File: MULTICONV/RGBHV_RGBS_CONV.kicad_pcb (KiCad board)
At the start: 2 copper layers, 100 x 100 mm, 111 parts, among them J1 DIGITAL RGB, J10 AUDIO1, J11 RGBHV_2, J12 AUDIO2, J15 RGBS_OUT1, J16 RGBS_OUT2, J17 VIN, J2 VGA DB15, J3 ANALOG RGB DA15, J4 X1, J5 DIGITAL_RGBHV_1, J6 ANALOG RGB, J7 DIGITAL_RGBHV_2, J8 SWITCHER, J9 RGBHV_1, U1 OUT_GND_IN_3.3V, U2 74HC86, U3 OUT_IN_GND_3.3V, U4 IN_OUT_GND_3.3V

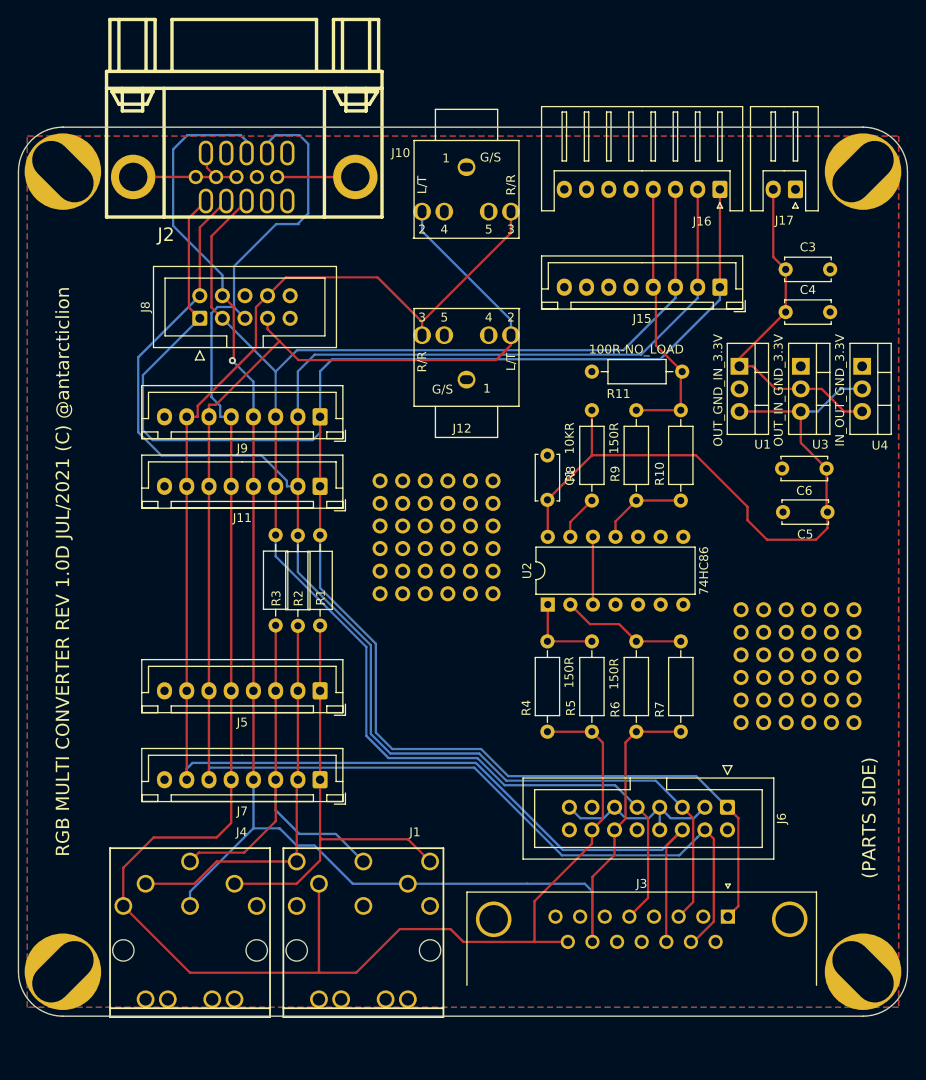
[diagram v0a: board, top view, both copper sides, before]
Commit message: Rev1.5 リリース候補
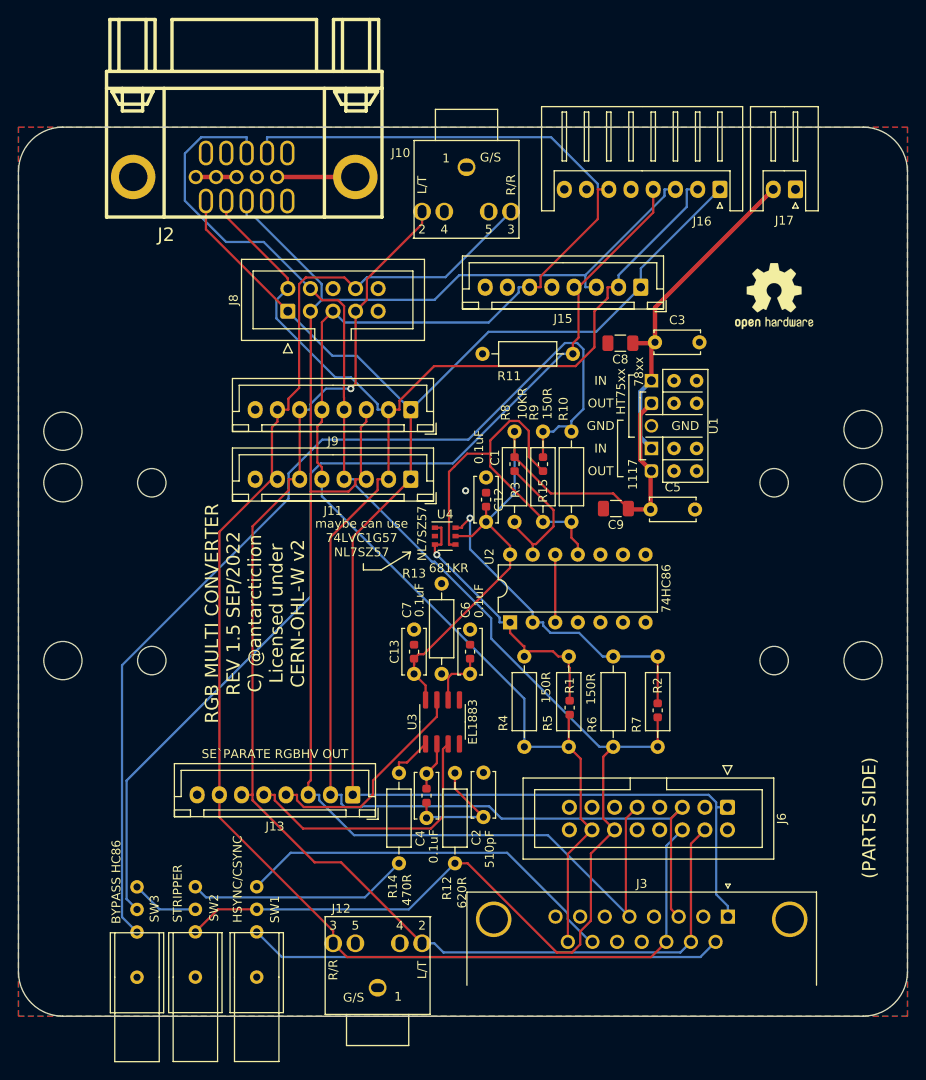
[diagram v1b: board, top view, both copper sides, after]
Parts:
- removed J1: DIGITAL RGB, ryuk_lib:DIN 8 PCB
- removed J4: X1, ryuk_lib:DIN_6_PCB
- removed J5: DIGITAL_RGBHV_1, Connector_JST:JST_XH_B8B-XH-A_1x08_P2.50mm_Vertical
- removed J7: DIGITAL_RGBHV_2, Connector_JST:JST_XH_B8B-XH-A_1x08_P2.50mm_Vertical
- removed PIN01 (x2), PIN02 (x2), PIN03 (x2), PIN04 (x2), PIN05 (x2), PIN06 (x2), PIN07 (x2), PIN08 (x2), PIN09 (x2), PIN10 (x2), PIN11 (x2), PIN12 (x2), PIN13 (x2), PIN14 (x2), PIN15 (x2), PIN16 (x2), PIN17 (x2), PIN18 (x2), PIN19 (x2), PIN20 (x2), PIN21 (x2), PIN22 (x2), PIN23 (x2), PIN24 (x2), PIN25 (x2), PIN26 (x2), PIN27 (x2), PIN28 (x2), PIN29 (x2), PIN30 (x2), PIN31 (x2), PIN32 (x2), PIN33 (x2), PIN34 (x2), PIN35 (x2), PIN36 (x2): Pin_2.54, ryuk_lib:Pin_2.54
- added C10: 0.1uF, Capacitor_SMD:C_0603_1608Metric, F.Cu at (95.9, 137.2)
- added C11: 0.1uF, Capacitor_SMD:C_0603_1608Metric, F.Cu at (100.8, 121.0)
- added C12: 0.1uF, Capacitor_SMD:C_0603_1608Metric, F.Cu at (102.6, 103.9)
- added C13: 0.1uF, Capacitor_SMD:C_0603_1608Metric, F.Cu at (94.5, 121.0)
- added C2: 510pF, Capacitor_THT:C_Disc_D5.0mm_W2.5mm_P5.00mm, F.Cu at (102.3, 139.6)
- added C7: 0.1uF, Capacitor_THT:C_Disc_D5.0mm_W2.5mm_P5.00mm, F.Cu at (94.5, 118.5)
- added C8: 10uF, Capacitor_SMD:C_1206_3216Metric, F.Cu at (117.7, 86.3)
- added C9: 10uF, Capacitor_SMD:C_1206_3216Metric, F.Cu at (117.2, 104.9)
- added H10: M4, MountingHole:MountingHole_4.3mm_M4, F.Cu at (55.0, 122.0)
- added H11: M4, MountingHole:MountingHole_4.3mm_M4, F.Cu at (145.0, 102.0)
- added H12: M4, MountingHole:MountingHole_4.3mm_M4, F.Cu at (145.0, 122.0)
- added H13: M4, MountingHole:MountingHole_4.3mm_M4, F.Cu at (55.0, 96.2)
- added H14: M4, MountingHole:MountingHole_4.3mm_M4, F.Cu at (145.0, 96.0)
- added H5: M3, MountingHole:MountingHole_3.2mm_M3, F.Cu at (135.0, 102.0)
- added H6: M3, MountingHole:MountingHole_3.2mm_M3, F.Cu at (65.0, 102.0)
- added H7: M3, MountingHole:MountingHole_3.2mm_M3, F.Cu at (135.0, 122.0)
- added H8: M3, MountingHole:MountingHole_3.2mm_M3, F.Cu at (65.0, 122.0)
- added H9: M4, MountingHole:MountingHole_4.3mm_M4, F.Cu at (55.0, 102.0)
- added J13: SE`PARATE RGBHV OUT, Connector_JST:JST_XH_B8B-XH-A_1x08_P2.50mm_Vertical, F.Cu at (87.6, 137.1)
- added R12: 620R, Resistor_THT:R_Axial_DIN0207_L6.3mm_D2.5mm_P10.16mm_Horizontal, F.Cu at (99.1, 144.8)
- added R13: 681KR, Resistor_THT:R_Axial_DIN0207_L6.3mm_D2.5mm_P10.16mm_Horizontal, F.Cu at (97.6, 123.5)
- added R14: 470R, Resistor_THT:R_Axial_DIN0207_L6.3mm_D2.5mm_P10.16mm_Horizontal, F.Cu at (92.8, 144.8)
- added R15: 150R, Resistor_SMD:R_0603_1608Metric, F.Cu at (109.0, 99.9)
- added REF**: OSHW-Logo2_9.8x8mm_SilkScreen, Symbol:OSHW-Logo2_9.8x8mm_SilkScreen, B.Cu at (135.0, 81.0)
- added REF**: OSHW-Logo2_9.8x8mm_SilkScreen, Symbol:OSHW-Logo2_9.8x8mm_SilkScreen, F.Cu at (135.0, 81.0)
- added SW1: HSYNC/CSYNC, ryuk_lib:2MS1T1B4M7QES, F.Cu at (76.8, 157.6)
- added SW2: STRIPPER, ryuk_lib:2MS1T1B4M7QES, F.Cu at (69.9, 157.6)
- added SW3: BYPASS HC86, ryuk_lib:2MS1T1B4M7QES, F.Cu at (63.3, 157.6)
- H1, H2, H3, H4: footprint MountingHole:MountingHole_4.3mm_M4_Pad -> MountingHole:MountingHole_4.3mm_M4
- R1, R2: footprint Resistor_THT:R_Axial_DIN0207_L6.3mm_D2.5mm_P10.16mm_Horizontal -> Resistor_SMD:R_0603_1608Metric
- R3: value 150R -> 10KR; footprint Resistor_THT:R_Axial_DIN0207_L6.3mm_D2.5mm_P10.16mm_Horizontal -> Resistor_SMD:R_0603_1608Metric
- U1: value OUT_GND_IN_3.3V -> 3V3_REG; footprint Package_TO_SOT_THT:TO-220-3_Vertical -> ryuk_lib:PIN_Unified_LDO
- U3: value OUT_IN_GND_3.3V -> EL1883; footprint Package_TO_SOT_THT:TO-220-3_Vertical -> Package_SO:SOIC-8_3.9x4.9mm_P1.27mm
- U4: value IN_OUT_GND_3.3V -> NL7SZ57; footprint Package_TO_SOT_THT:TO-220-3_Vertical -> Package_SO:TSOP-6_1.65x3.05mm_P0.95mm
- moved C4 69.8 mm to (95.9, 139.7), turned to 90 degrees
- moved J12 69.1 mm to (90.4, 161.8)
- moved U3 56.8 mm to (97.7, 128.9), turned to 90 degrees
- moved U4 50.6 mm to (98.0, 108.0), turned to 0 degrees
- moved C6 46.3 mm to (100.8, 123.5), turned to 90 degrees
- moved R2 41.6 mm to (121.9, 127.6)
- moved R3 32.4 mm to (105.8, 99.9)
- moved R1 29.6 mm to (112.0, 127.3), turned to 270 degrees
- moved C5 19.9 mm to (121.1, 105.0), turned to 0 degrees
- moved C3 16.8 mm to (121.6, 86.2)
- moved R10 12.5 mm to (112.2, 106.4)
- moved R11 12.5 mm to (102.2, 87.5)
- moved U1 12.0 mm to (121.2, 95.6), turned to 90 degrees
- moved R9 10.8 mm to (109.0, 106.4)
- moved J11 10.2 mm to (94.1, 101.6)
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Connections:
- C4 pad 1: Net-(C3-Pad1) -> Net-(C10-Pad1)
- C4 pad 2: GND -> Net-(C10-Pad2)
- C6 pad 1: +3V3 -> Net-(C11-Pad1)
- J15 pad 5: Net-(J15-Pad5) -> (no net)
- J15 pad 6: Net-(J15-Pad6) -> VSYNC
- J15 pad 7: Net-(J15-Pad7) -> (no net)
- J16 pad 5: Net-(J16-Pad5) -> (no net)
- J16 pad 6: Net-(J16-Pad6) -> VSYNC
- J16 pad 7: Net-(J16-Pad7) -> (no net)
- J2 pad 12: Net-(J2-Pad12) -> (no net)
- J2 pad 15: Net-(J2-Pad15) -> (no net)
- J2 pad 4: Net-(J2-Pad4) -> (no net)
- J2 pad 5: Net-(J2-Pad5) -> (no net)
- J2 pad 9: Net-(J2-Pad9) -> (no net)
- J3 pad 13: Net-(J3-Pad13) -> (no net)
- J3 pad 14: HSYNC -> Net-(J3-Pad14)
- J3 pad 7: Net-(J3-Pad7) -> (no net)
- J6 pad 10: Net-(J6-Pad10) -> (no net)
- J6 pad 13: Net-(J6-Pad13) -> (no net)
- J6 pad 16: Net-(J6-Pad16) -> (no net)
- J6 pad 2: Net-(J6-Pad2) -> (no net)
- R1 pad 1: DIGITAL_R -> Net-(R1-Pad1)
- R1 pad 2: R -> VSYNC
- R10 pad 2: CSYNC -> Net-(R10-Pad2)
- R2 pad 1: DIGITAL_G -> HSYNC
- R2 pad 2: G -> Net-(R2-Pad2)
- R3 pad 1: DIGITAL_B -> Net-(R3-Pad1)
- R3 pad 2: B -> +3V3
- R4 pad 2: Net-(R4-Pad2) -> Net-(R1-Pad1)
- R5 pad 2: Net-(R4-Pad2) -> Net-(R1-Pad1)
- R6 pad 2: Net-(R6-Pad2) -> Net-(R2-Pad2)
- R7 pad 2: Net-(R6-Pad2) -> Net-(R2-Pad2)
- R8 pad 1: Net-(R8-Pad1) -> Net-(R3-Pad1)
- R9 pad 2: CSYNC -> Net-(R10-Pad2)
- U2 pad 1: Net-(R4-Pad2) -> Net-(R1-Pad1)
- U2 pad 13: Net-(R8-Pad1) -> Net-(R3-Pad1)
- U2 pad 2: Net-(R6-Pad2) -> Net-(R2-Pad2)
- U2 pad 6: Net-(U2-Pad6) -> (no net)
- U2 pad 8: Net-(U2-Pad8) -> (no net)
- U3 pad 1: GND -> Net-(R14-Pad2)
- U3 pad 2: Net-(C3-Pad1) -> Net-(C10-Pad2)
- U3 pad 3: +3V3 -> Net-(J13-Pad5)
- U4 pad 1: GND -> Net-(R1-Pad1)
- U4 pad 2: +3V3 -> GND
- U4 pad 3: Net-(C3-Pad1) -> Net-(R1-Pad1)
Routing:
- net Net-(R10-Pad2): track 0.00 -> 115.7 mm
- net CSYNC: track 31.3 -> 115.9 mm
- net Net-(J3-Pad9): track 0.00 -> 53.5 mm
- net DIGITAL_R: track 50.6 -> 0.00 mm
- net DIGITAL_B: track 49.2 -> 0.00 mm
- net DIGITAL_G: track 44.6 -> 0.00 mm
- net Net-(J3-Pad14): track 0.00 -> 43.9 mm
- net Net-(R2-Pad2): track 0.00 -> 38.0 mm, vias 0 -> 1
- net VSYNC: track 210.5 -> 176.0 mm
- net Net-(R10-Pad1): track 10.0 -> 44.1 mm
- net Net-(R1-Pad1): track 0.00 -> 31.1 mm, vias 0 -> 1
- net GND: track 44.4 -> 13.4 mm, vias 0 -> 1
- net Net-(J13-Pad5): track 0.00 -> 31.0 mm
- net AUDIO_L: track 179.6 -> 148.6 mm, vias 0 -> 1
- net R: track 212.5 -> 182.8 mm
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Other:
- board text added: "A_L"
- board text added: "A_R"
- board text added: "B"
- board text added: "G"
- board text added: "H"
- board text added: "IDC EXTRA DA15 CONNECTOR"
- board text added: "ISL59885 Configuration R13 - do not use C6 - 0.056uF"
- board text added: "Maybe can use 74HC86 74AC86 74AHC86"
- board text added: "R"
- board text added: "RGB MULTI CONVERTER REV 1.5 SEP/2022 C) @antarcticlion Licensed under CERN-OHL-W v2"
- board text added: "S"
- board text added: "SYNC SEPARATER OUTPUT"
- board text added: "V"
- board text added: "maybe can use 74LVC1G57 NL7SZ57"
- board text removed: "1117"
- board text removed: "48033"
- board text removed: "7533-1"
- board text removed: "RGB MULTI CONVERTER REV 1.0D JUL/2021 (C) @antarcticlion"
